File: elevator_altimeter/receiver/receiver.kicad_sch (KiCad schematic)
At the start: 39 parts, among them Q1 TP0606, Q2 VN2210N, SW1 UserSW, SW2 PWR_SW, U1 ATmega32U4-A, U2 5631AH-S_3digit_7segment_disp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, U3 NRF24L01_Breakout, U4 PQ070XNA1ZPH

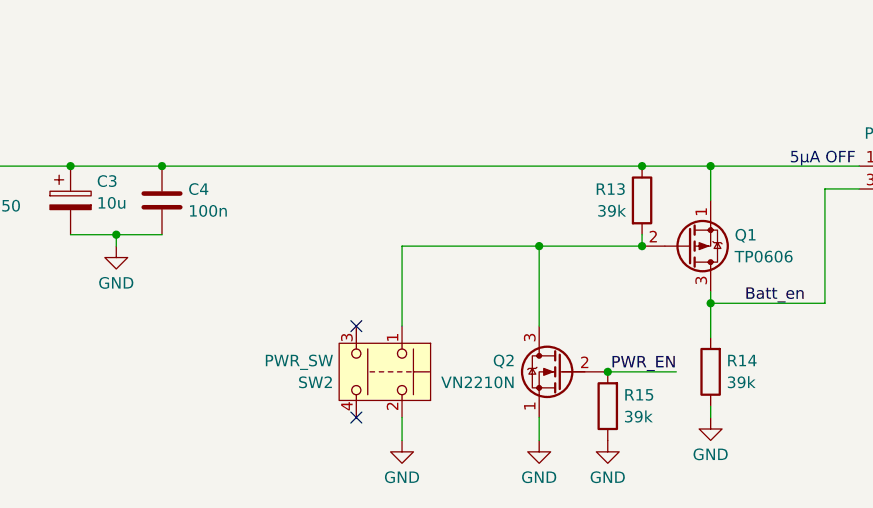
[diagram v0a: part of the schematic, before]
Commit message: a
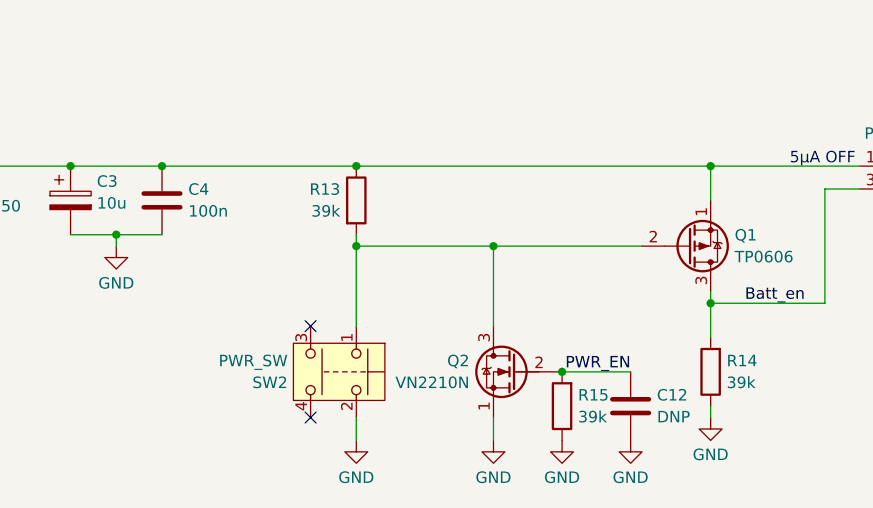
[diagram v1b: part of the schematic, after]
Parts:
- added C12: DNP, symbol Device:C
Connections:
- net GND: now also C12.2
- net PWR_EN: now also C12.1
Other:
- moved on the sheet: Q2, R13, R15, SW2
